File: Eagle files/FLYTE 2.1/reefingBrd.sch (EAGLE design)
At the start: 37 parts, among them U1 RASPBERRY_PICOSMD, U2 GY-521MPU6050, U7 IRF540NPBF

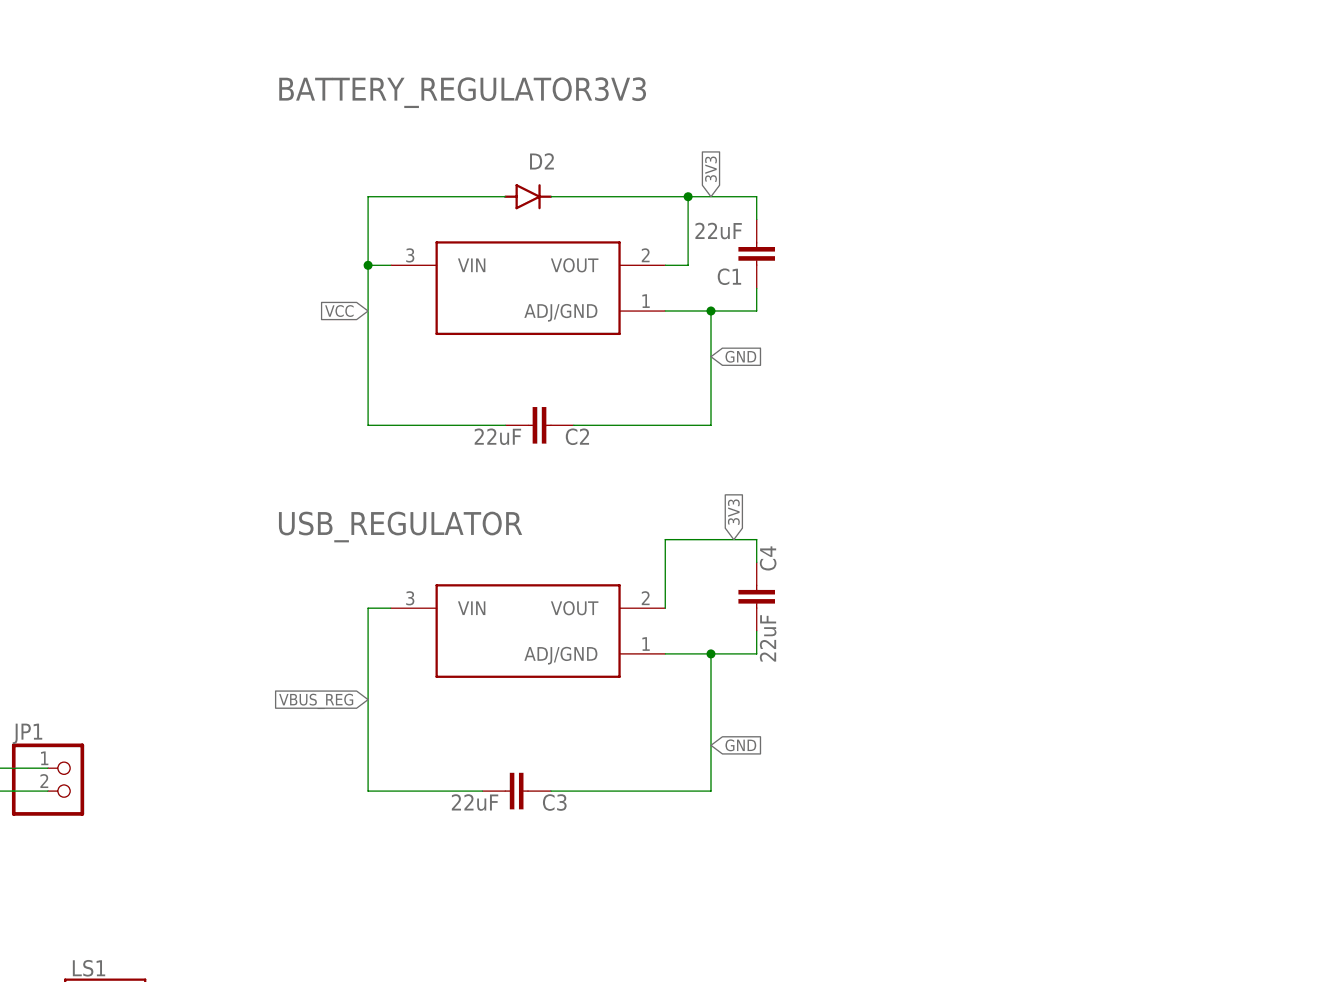
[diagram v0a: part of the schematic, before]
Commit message: reefing
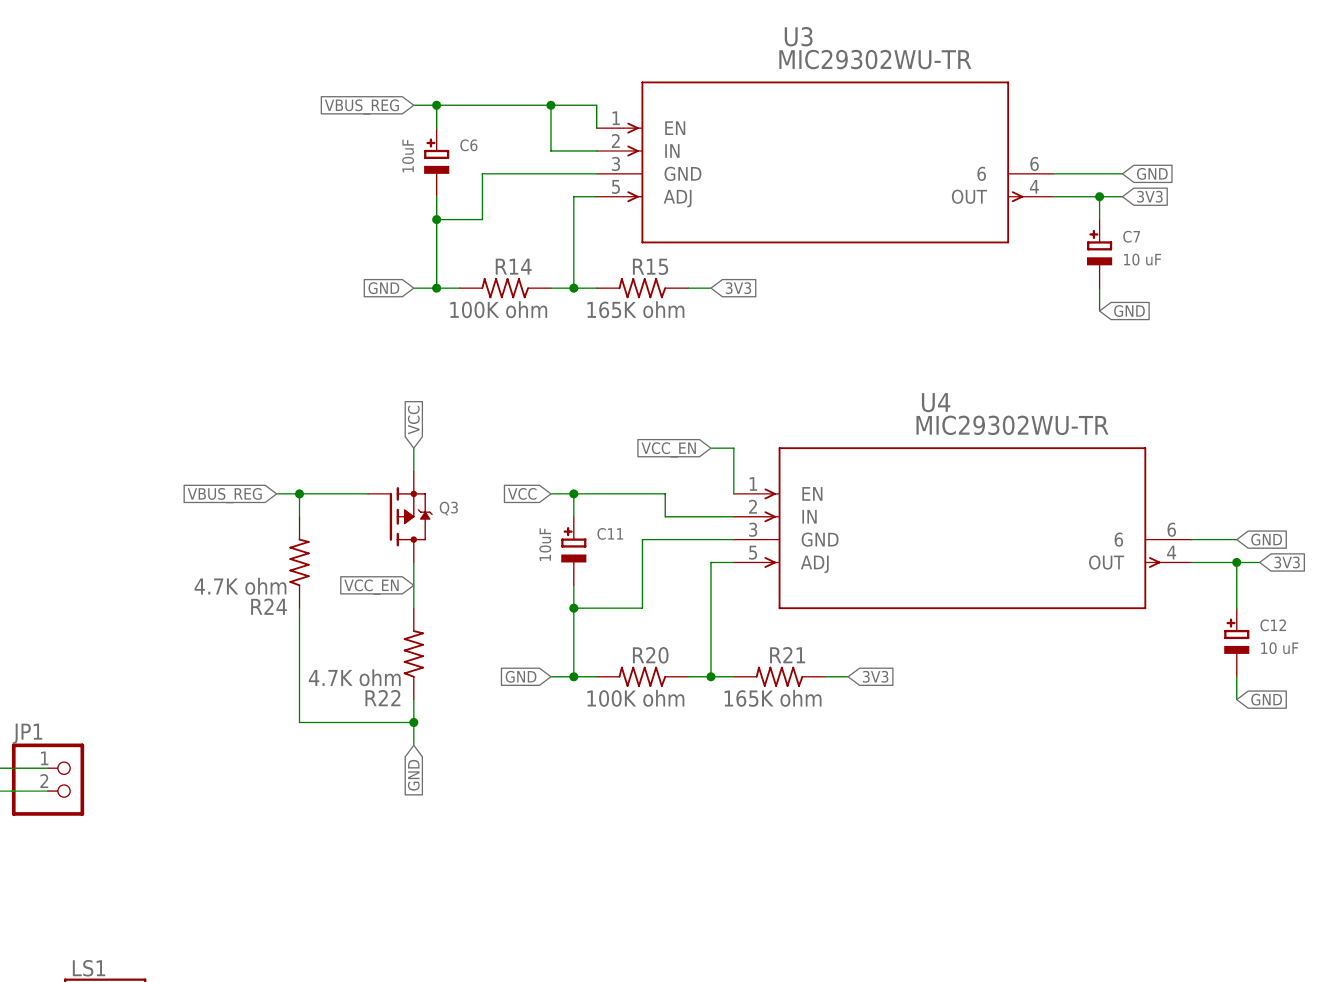
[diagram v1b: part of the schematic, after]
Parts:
- removed BATTERY_REGULATOR3V3, USB_REGULATOR: AMS1117-3.3, AMS1117-3.3:AMS1117-3.3
- removed C1, C2, C3, C4: 22uF, SparkFun-Capacitors:22UF-0805-6.3V-20%
- removed D2: 1N4004, diode:1N4004
- added C11, C6: 10uF, microbuilder:CAP_TANTALUMA/3216_WAVE
- added C12, C7: 10 uF, microbuilder:CAP_TANTALUMA/3216_WAVE
- added Q3: (no value), microbuilder:MOSFET-PWIDE
- added R14, R20: 100K ohm, rcl:R-US_R0805
- added R15, R21: 165K ohm, rcl:R-US_R0805
- added R22, R24: 4.7K ohm, rcl:R-US_R0805
- added U3, U4: MIC29302WU-TR, MIC29302WU:MIC29302WU-TR
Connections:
- new net N$10: R14.1, R15.2, U3.ADJ
- new net N$3: R20.1, R21.2, U4.ADJ
- new net VCC_EN: Q3.D, R22.2, U4.EN
- net 3V3: now also C12.+, C7.+, R15.1, R21.1, U3.OUT, U4.OUT; no longer BATTERY_REGULATOR3V3.VOUT, C1.2, C4.1, D2.C, USB_REGULATOR.VOUT
- net GND: now also C11.-, C12.-, C6.-, C7.-, R14.2, R20.2, R22.1, R24.1, U3.6, U3.GND, U4.6, U4.GND; no longer BATTERY_REGULATOR3V3.ADJ/GND, C1.1, C2.1, C3.1, C4.2, USB_REGULATOR.ADJ/GND
- net VBUS_REG: now also C6.+, Q3.G, R24.2, U3.EN, U3.IN; no longer C3.2, USB_REGULATOR.VIN
- net VCC: now also C11.+, Q3.S, U4.IN; no longer BATTERY_REGULATOR3V3.VIN, C2.2, D2.A
